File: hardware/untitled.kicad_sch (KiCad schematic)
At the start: 13 parts

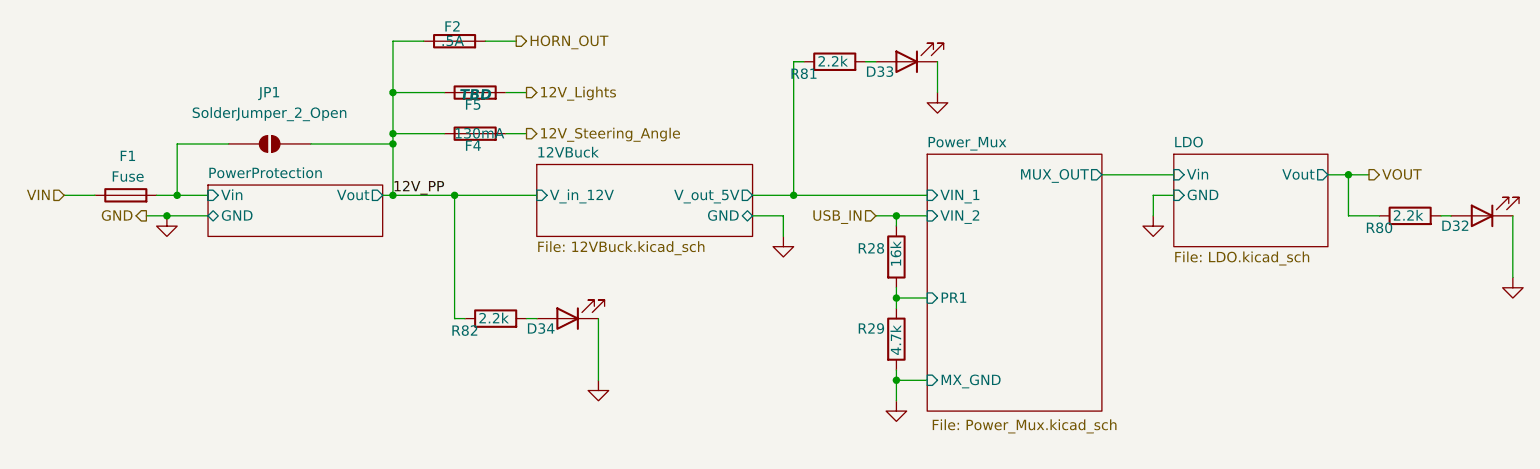
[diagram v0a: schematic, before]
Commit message: rawr
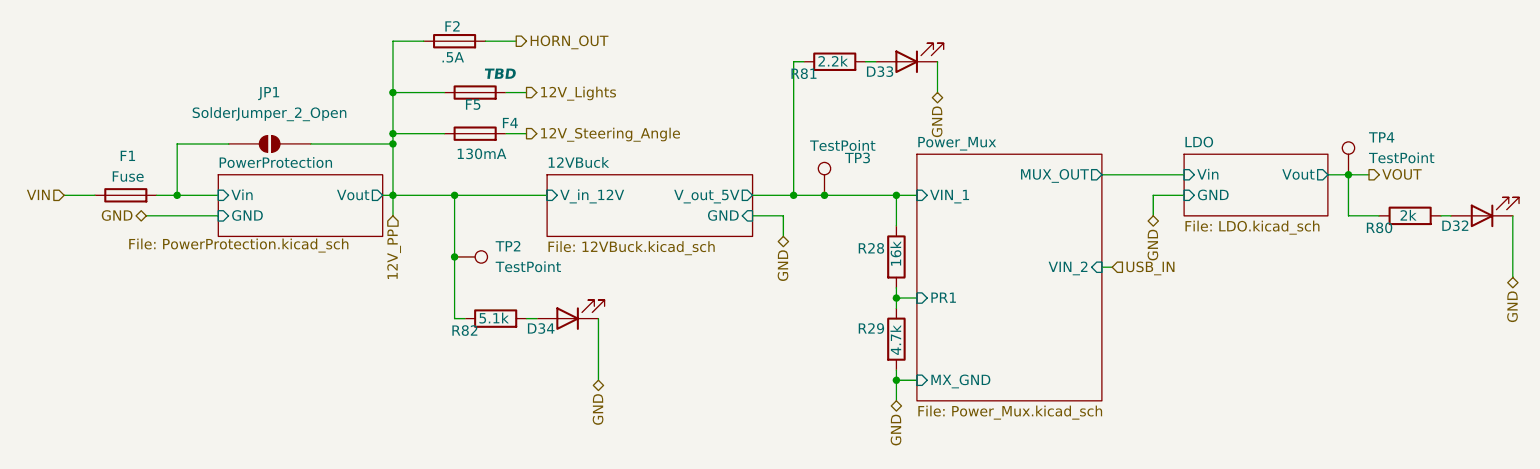
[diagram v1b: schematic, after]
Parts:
- added TP2, TP3, TP4: TestPoint, symbol Connector:TestPoint
- R80: value 2.2k -> 2k
- R82: value 2.2k -> 5.1k
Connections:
- net 12VBuck/V_out_5V: now also R28.1, TP3.1
- net 12V_PP: now also TP2.1
- net USB_IN: no longer R28.1
- net VOUT: now also TP4.1
